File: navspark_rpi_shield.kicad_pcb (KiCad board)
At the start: 2 copper layers, 45 x 42 mm, 7 parts, among them P1 CONN_02X13, P2 CONN_01X13, P3 CONN_01X12

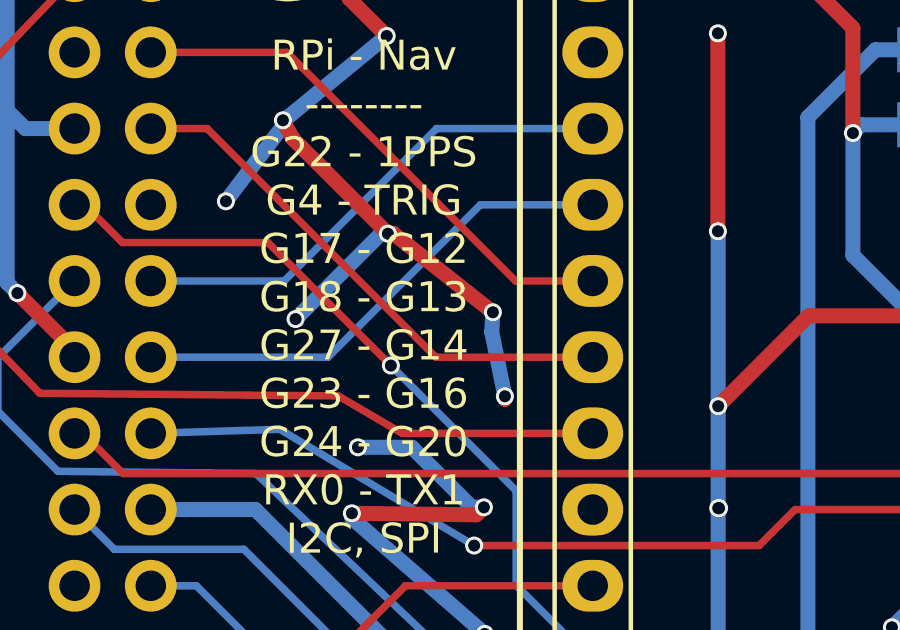
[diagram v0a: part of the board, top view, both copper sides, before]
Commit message: small changes
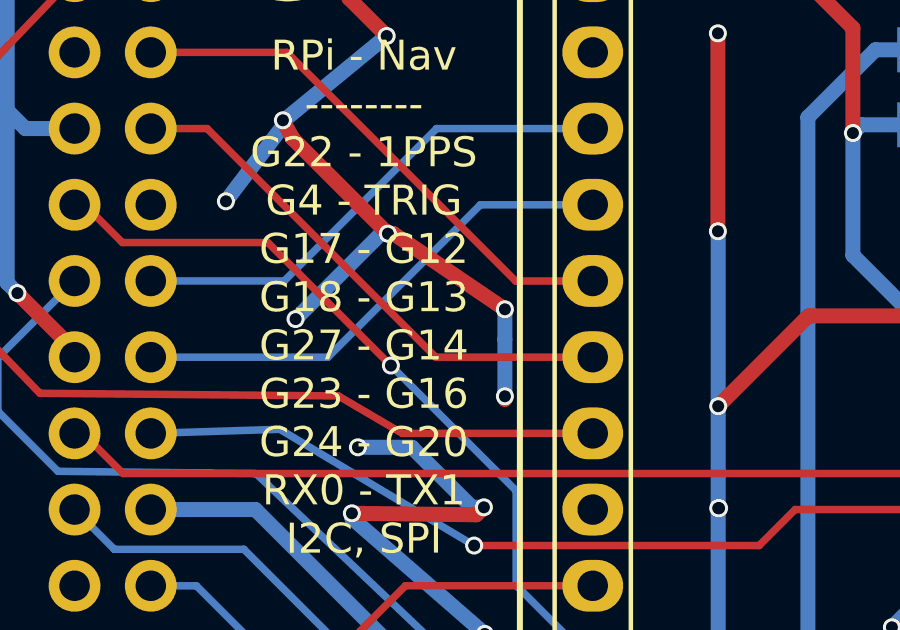
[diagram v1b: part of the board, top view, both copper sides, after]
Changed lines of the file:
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@@
   (segment (start 119.5 121.7) (end 119.5 121.81) (width 0.5) (layer F.Cu) (net 2))
   (via (at 119.5 121.7) (size 0.6) (drill 0.4) (layers F.Cu B.Cu) (net 2))
-  (segment (start 119.06 119.55) (end 119.5 121.7) (width 0.5) (layer B.Cu) (net 2))
-  (segment (start 119.1 118.9) (end 119.06 119.55) (width 0.5) (layer B.Cu) (net 2))
-  (via (at 119.1 118.9) (size 0.6) (drill 0.4) (layers F.Cu B.Cu) (net 2))
-  (segment (start 115.79 116.28) (end 119.1 118.9) (width 0.5) (layer F.Cu) (net 2))
+  (segment (start 119.5 119.8) (end 119.5 121.7) (width 0.5) (layer B.Cu) (net 2))
+  (segment (start 119.5 118.8) (end 119.5 119.8) (width 0.5) (layer B.Cu) (net 2))
+  (via (at 119.5 118.8) (size 0.6) (drill 0.4) (layers F.Cu B.Cu) (net 2))
+  (segment (start 115.79 116.28) (end 119.5 118.8) (width 0.5) (layer F.Cu) (net 2))
   (segment (start 133.12 119.02) (end 129.62 119.02) (width 0.5) (layer F.Cu) (net 2))
   (segment (start 126.61 125.43) (end 126.64 125.43) (width 0.5) (layer F.Cu) (net 2))
@@
     (connect_pads (clearance 0.508))
     (min_thickness 0.254)
-    (fill (arc_segments 16) (thermal_gap 0.508) (thermal_bridge_width 0.508))
+    (fill yes (arc_segments 16) (thermal_gap 0.508) (thermal_bridge_width 0.508))
     (polygon
       (pts
@@
     (connect_pads (clearance 0.508))
     (min_thickness 0.254)
-    (fill (arc_segments 16) (thermal_gap 0.508) (thermal_bridge_width 0.508))
+    (fill yes (arc_segments 16) (thermal_gap 0.508) (thermal_bridge_width 0.508))
     (polygon
       (pts
